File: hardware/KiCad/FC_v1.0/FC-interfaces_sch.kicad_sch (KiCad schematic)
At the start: 39 parts, among them J10 PAD_OUT, J11 PAD_OUT, J12 PAD_OUT_Mini, J13 PAD_OUT_Mini, J2 MEM2061-01-188-00-A, J3 USB4105-GF-A, J4 Conn_ARM_SWD_TagConnect_TC203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, J5 SM06B-GHS-TB, J6 SM04B-GHS-TB, J7 SM06B-GHS-TB, J8 SM06B-GHS-TB, J9 SM04B-GHS-TB, Q1 AO3400A, U8 USBLC6-2SC6

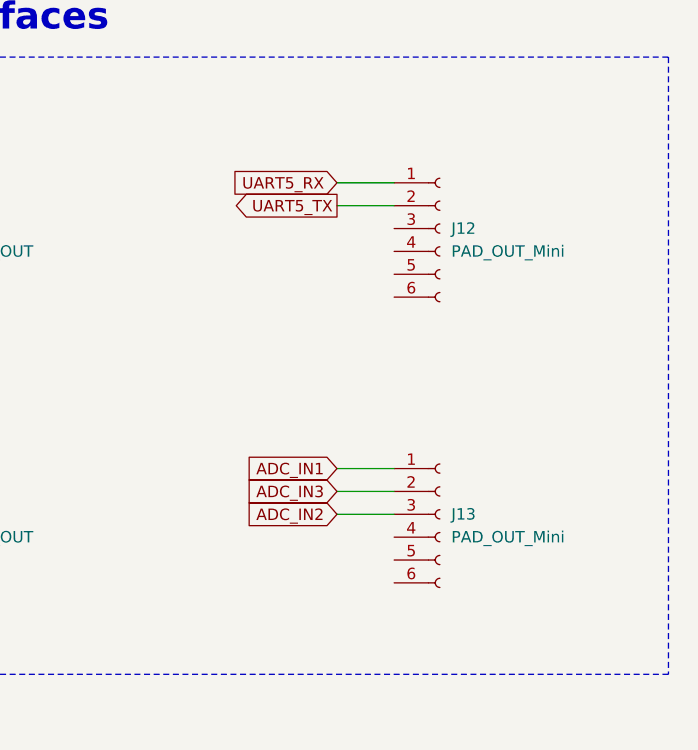
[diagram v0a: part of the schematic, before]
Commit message: Top/Bot pours
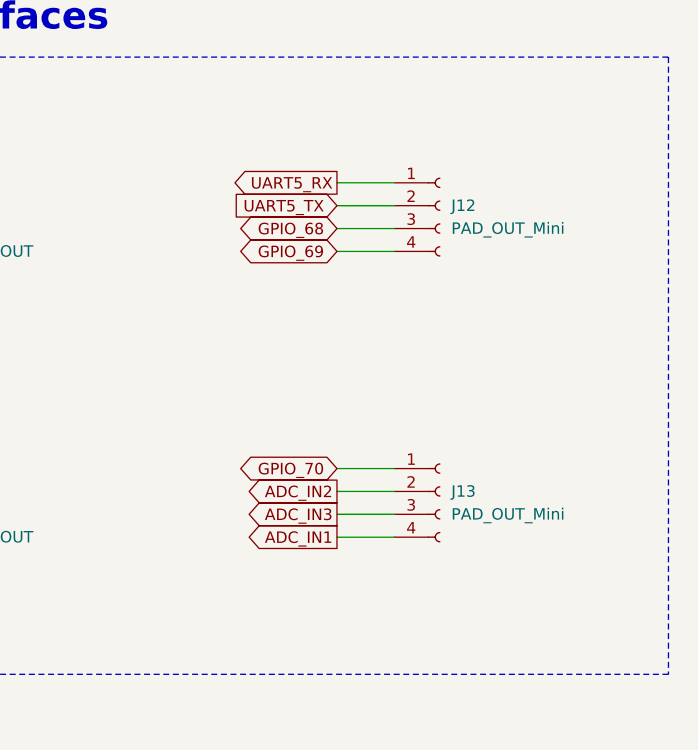
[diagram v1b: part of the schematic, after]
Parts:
- removed J12, J13: PAD_OUT_Mini, FC-FootprintLib:Mini_Pad_out_1x6, symbol Connector:Conn_01x06_Socket
- added J12, J13: PAD_OUT_Mini, FC-FootprintLib:Pad_out_mini_1x4, symbol Connector:Conn_01x04_Socket
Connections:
- net ADC_IN1: now also J13.4 (Pin_4)
- net ADC_IN2: now also J13.2 (Pin_2)
- net ADC_IN3: now also J13.3 (Pin_3)
- net UART5_RX: now also J12.1 (Pin_1)
- net UART5_TX: now also J12.2 (Pin_2)
- new net GPIO_68: J12.3 (Pin_3)
- new net GPIO_69: J12.4 (Pin_4)
- new net GPIO_70: J13.1 (Pin_1)
